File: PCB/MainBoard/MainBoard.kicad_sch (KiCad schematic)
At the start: 17 parts, among them Q1 PT334-6C, SW1 PWR SWITCH, SW1 SW_DIP_x05, U1 LM393, U2 ESP32-WROOM-32

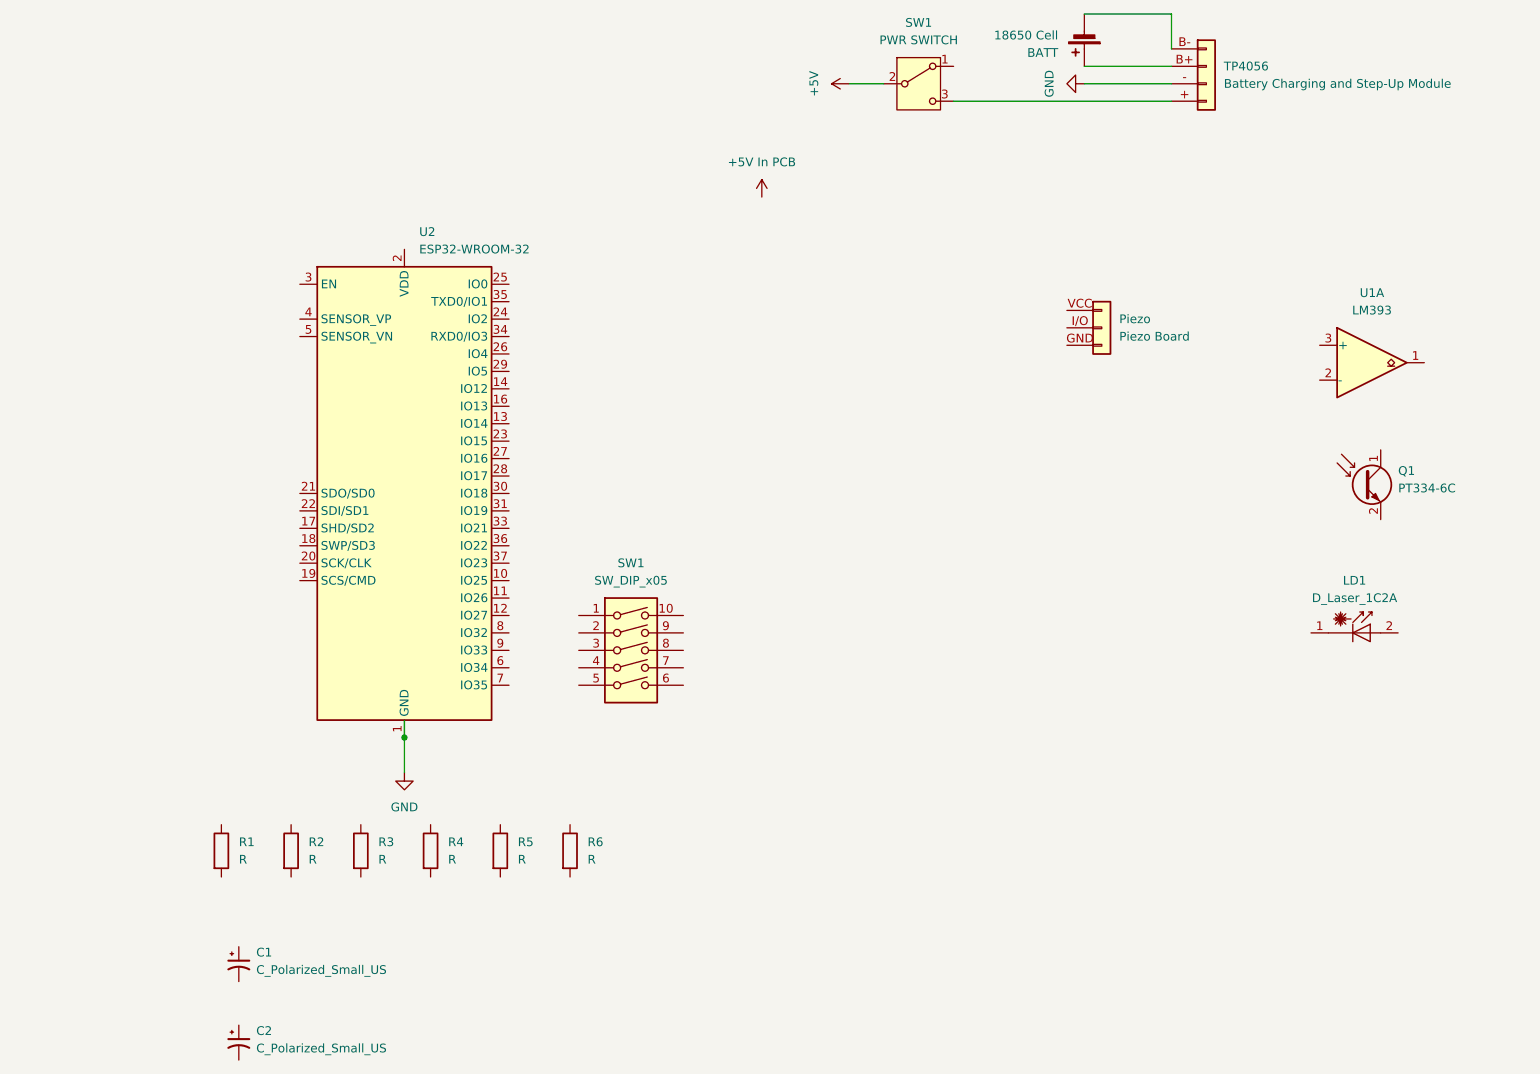
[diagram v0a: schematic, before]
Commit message: Iniital schematic (poor layout), and added additional functionality to the firmware
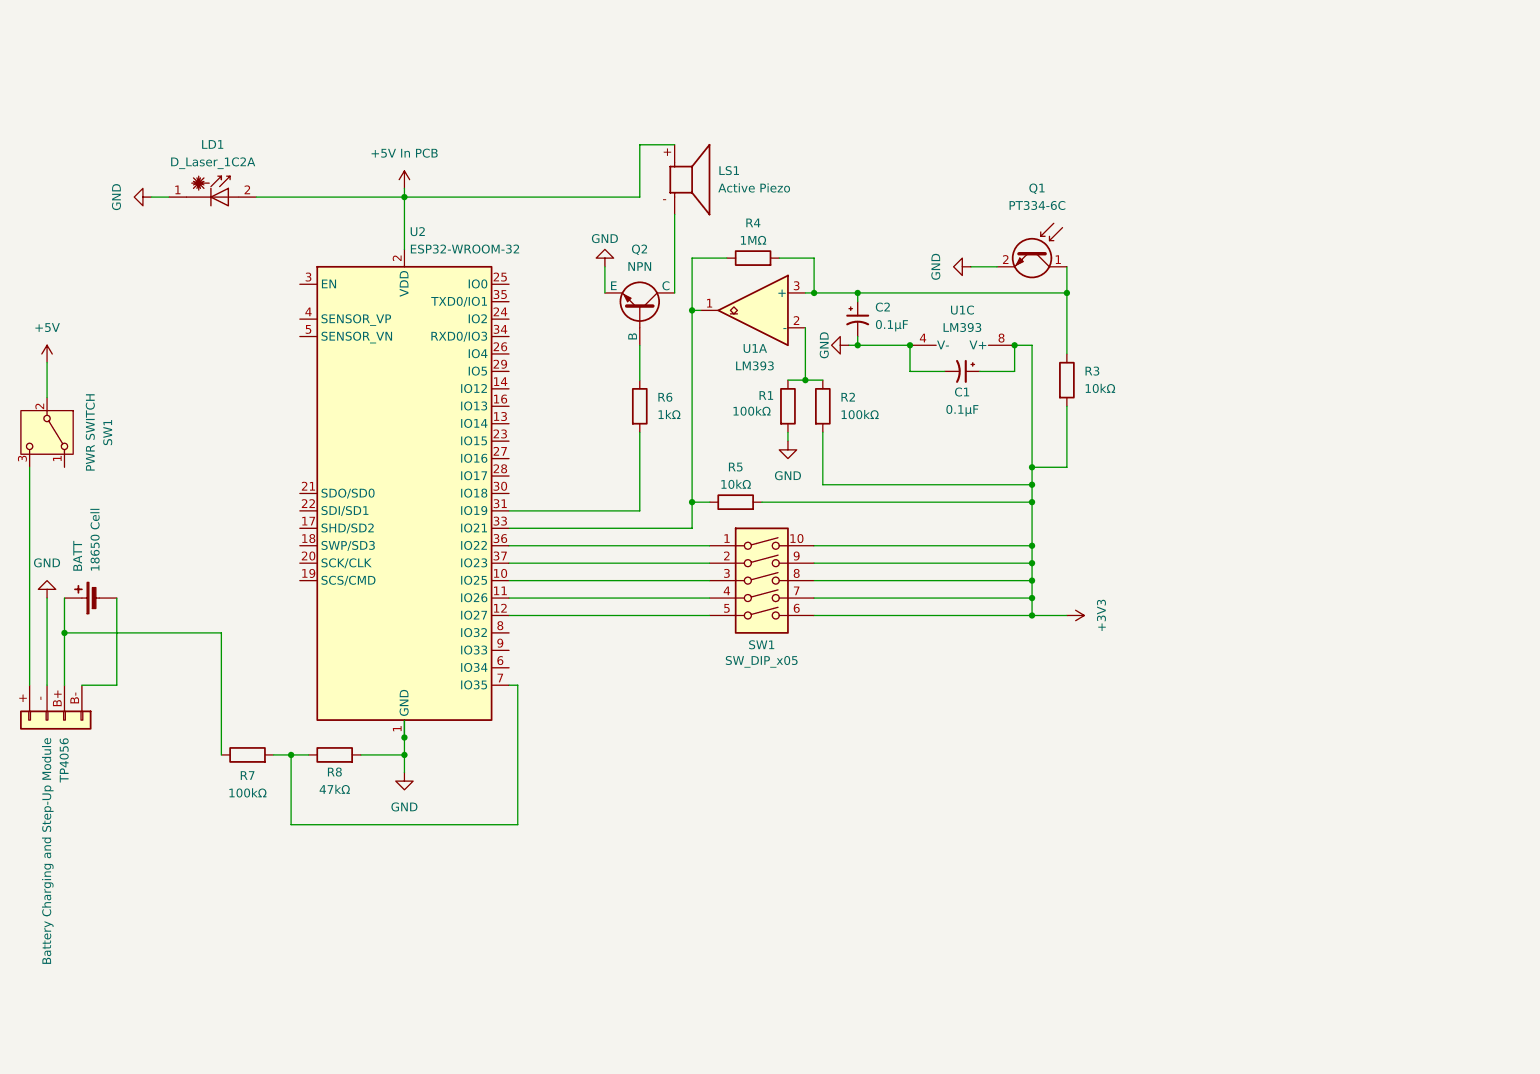
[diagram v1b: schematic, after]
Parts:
- removed Piezo: Piezo Board, symbol Connector_Generic:Conn_01x03
- added LS1: Active Piezo, CMI-1295IC-0585T:CUI_CMI-1295IC-0585T, symbol CMI-1295IC-0585T Piezo:CMI-1295IC-0585T
- added Q2: NPN, symbol Simulation_SPICE:NPN
- added R7: 100kΩ, symbol Device:R
- added R8: 47kΩ, symbol Device:R
- added unit 3 of U1
- C1, C2: value C_Polarized_Small_US -> 0.1µF
- R1, R2: value R -> 100kΩ
- R3, R5: value R -> 10kΩ
- R4: value R -> 1MΩ
- R6: value R -> 1kΩ
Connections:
- net +5V In PCB: now also LD1.2 (A), U2.2 (VDD), LS1.
- net GND: now also C1.2, C2.2, LD1.1 (K), Q1.2 (E), R1.2, Q2.3 (E), R8.2, U1.4 (V-)
- net +3V3: now reaches C1.1
- net +3V3: now also R2.2, R3.2, R5.2, SW1.10, SW1.6, SW1.7, SW1.8, SW1.9, U1.8 (V+)
- net at R1.1: now also R2.1, U1.2 (-)
- net at R5.1: now also R4.1, U1.1, U2.33 (IO21)
- net at Q1.1 (C): now also C2.1, R3.1, R4.2, U1.3 (+)
- net at U2.10 (IO25): now also SW1.3
- net at U2.11 (IO26): now also SW1.4
- net at U2.12 (IO27): now also SW1.5
- net at U2.31 (IO19): now also R6.2
- net at U2.36 (IO22): now also SW1.1
- net at U2.37 (IO23): now also SW1.2
- net at U2.7 (IO35): now also R7.2, R8.1
- net at R6.1: now also Q2.2 (B)
- net at BATT.1 (+), TP4056.B+ (Batt+): now also R7.1
- new net: LS1., Q2.1 (C)
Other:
- moved on the sheet: BATT, C1, C2, LD1, Q1, R1, R2, R3, R4, R5, R6, SW1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
